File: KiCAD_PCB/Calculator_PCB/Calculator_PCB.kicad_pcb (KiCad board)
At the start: 2 copper layers, 109 parts, among them J1 USB_B_Micro, SW1 SW_SPST, SW10 SW_SPST, SW11 SW_SPST, SW12 SW_SPST, SW13 SW_SPST, SW14 SW_SPST, SW15 SW_SPST, SW16 SW_SPST, SW17 SW_SPST, SW18 SW_SPST, SW19 SW_SPST, SW2 SW_SPST, SW20 SW_SPST, SW21 SW_SPST, SW22 SW_SPST, SW23 SW_SPST, SW24 SW_SPST, SW25 SW_SPST, SW26 SW_SPST, SW27 SW_SPST, SW28 SW_SPST, SW29 SW_SPST, SW3 SW_SPST, SW30 SW_SPST, SW31 SW_SPST, SW32 SW_SPST, SW33 SW_SPST, SW34 SW_SPST, SW35 SW_SPST, SW36 SW_SPST, SW37 SW_SPST, SW38 SW_SPST, SW39 SW_SPST, SW4 SW_SPST, SW40 SW_SPST, SW5 SW_SPST, SW6 SW_SPST, SW7 SW_SPST, SW8 SW_SPST, SW9 SW_SPST, U1 W25Q128JVS, U2 RP2040, U3 NCP1117-3.3_SOT223, X1 JTAG-CORTEX, Y1 ABLS-12.000MHZ-B4-T

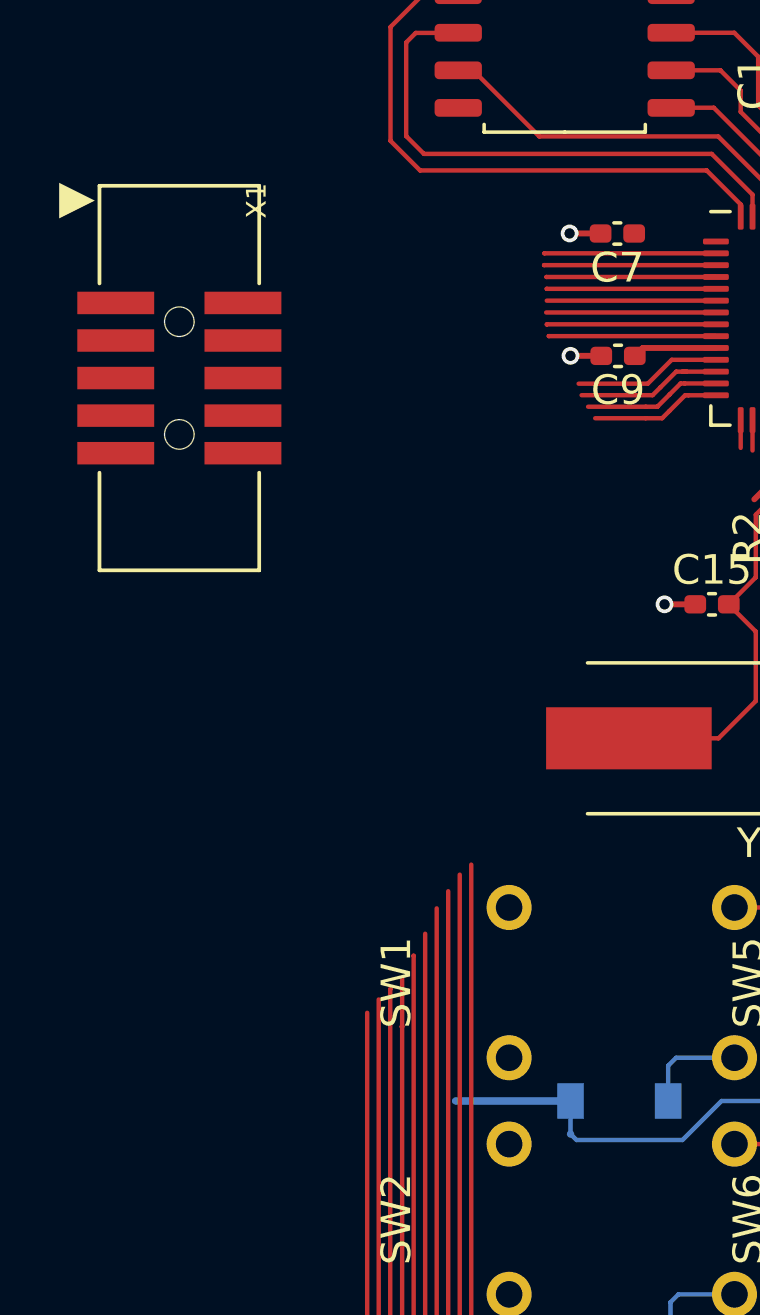
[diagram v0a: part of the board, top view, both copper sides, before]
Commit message: PCB Updates
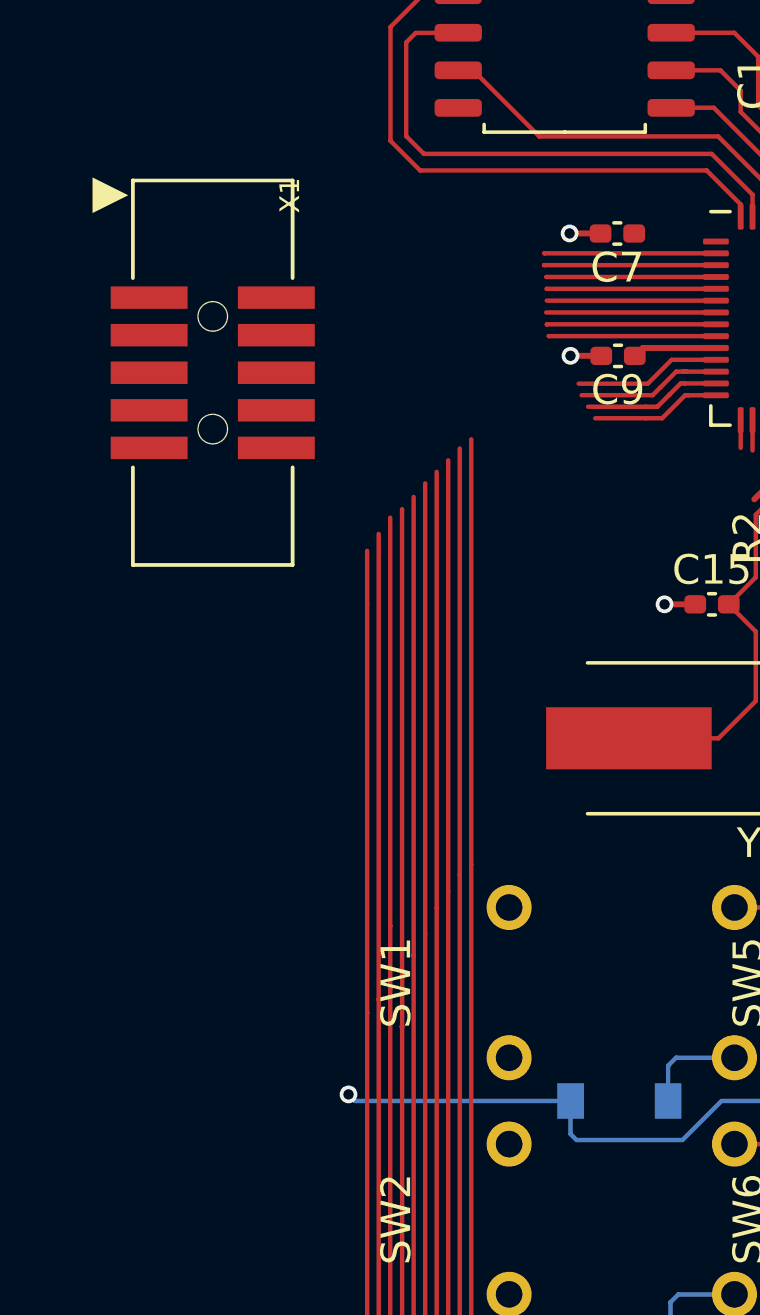
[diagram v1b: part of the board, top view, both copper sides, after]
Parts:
- moved X1 1.14 mm to (76.3, 91.4)
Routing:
- net /Col10: track 154.0 -> 169.9 mm
- net /Col9: track 141.7 -> 157.5 mm
- net /Col11: track 163.1 -> 178.8 mm
- net /Col12: track 175.7 -> 191.3 mm
- net /Col8: track 129.8 -> 145.3 mm
- net /Col7: track 114.0 -> 129.2 mm
- net /Col6: track 102.6 -> 117.3 mm
- net /Col5: track 90.3 -> 104.8 mm
- net /Col4: track 77.9 -> 92.3 mm
- net /Col3: track 65.3 -> 79.6 mm
- net /Row2: track 133.1 -> 136.8 mm, vias 0 -> 1
